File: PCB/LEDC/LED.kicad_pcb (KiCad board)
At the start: 2 copper layers, 70 x 70 mm, 38 parts, among them J1 Reset, J2 Wago, J3 TC2030-USB-NL-DS, J5 USB-C-Socket-H, SW1 Button, U1 ICS43434_MEMS_Mic, U2 IRMHF384, U6 ESP32-S3-MINI-1, U7 MD8942

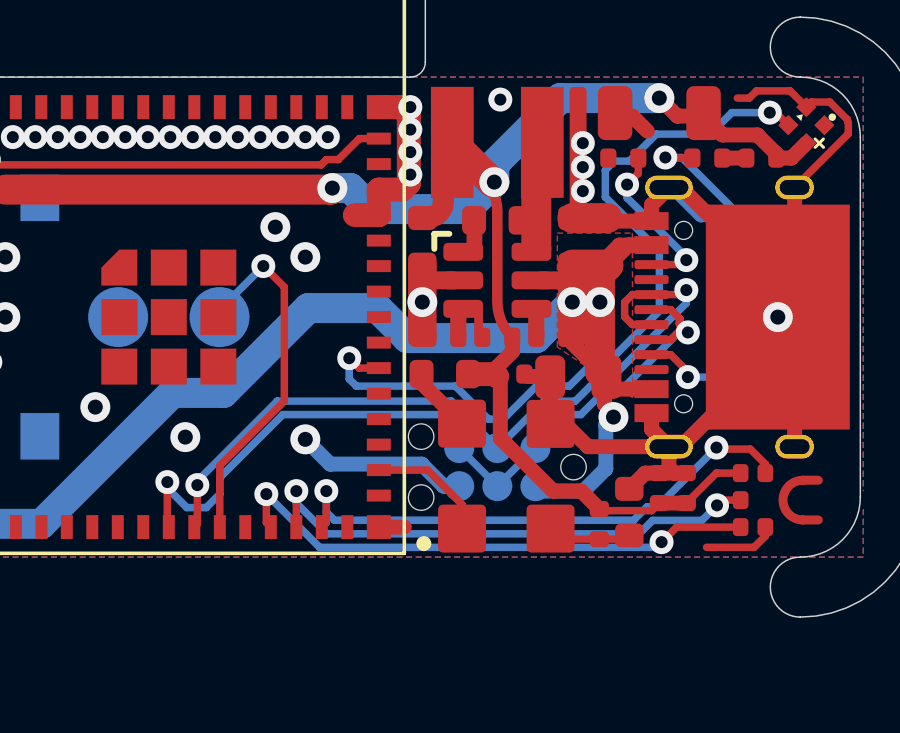
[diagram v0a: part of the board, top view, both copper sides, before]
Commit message: Tweak
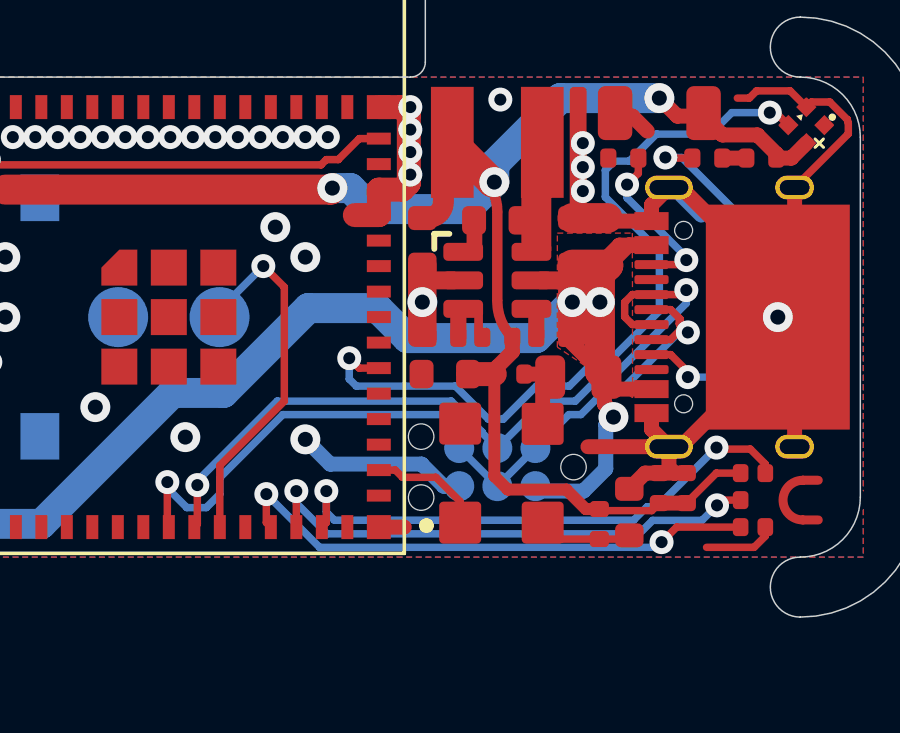
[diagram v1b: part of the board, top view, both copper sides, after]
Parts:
- moved U2 0.19 mm to (109.5, 105.2)
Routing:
- net GND: track 71.7 -> 68.0 mm
- net +3V3: track 52.6 -> 53.5 mm
- net Net-(U2-VCC): track 2.15 -> 2.99 mm
